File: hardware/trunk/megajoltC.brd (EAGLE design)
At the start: 79.9 x 63 mm, 116 parts, among them IC1 IC_FT230X-SSOP-16, IC2 MCP1826, IC3 MCP1826, J3 JUMPER_CLOSEDTHICK, U1 MCP1700, U11 TLV274, U12 PESDXS4UD, U18 MCP2551SO8, U4 ZXMS6004FF, U8 FAN8303, X1 MINI_USB_SHIELD, X3 MOLEX_MINIFIT-22

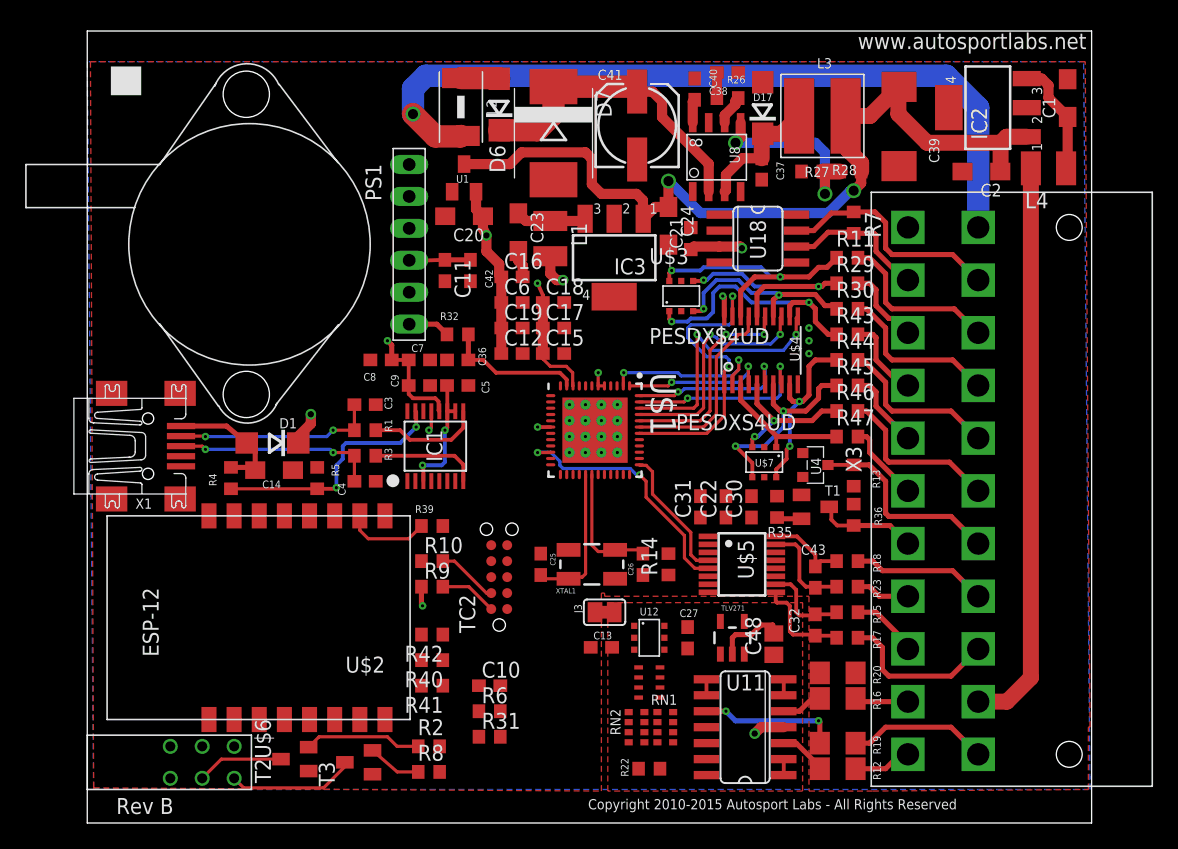
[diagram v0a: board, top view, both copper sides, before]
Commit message: Schematic, second draft complete
Also added gitignore
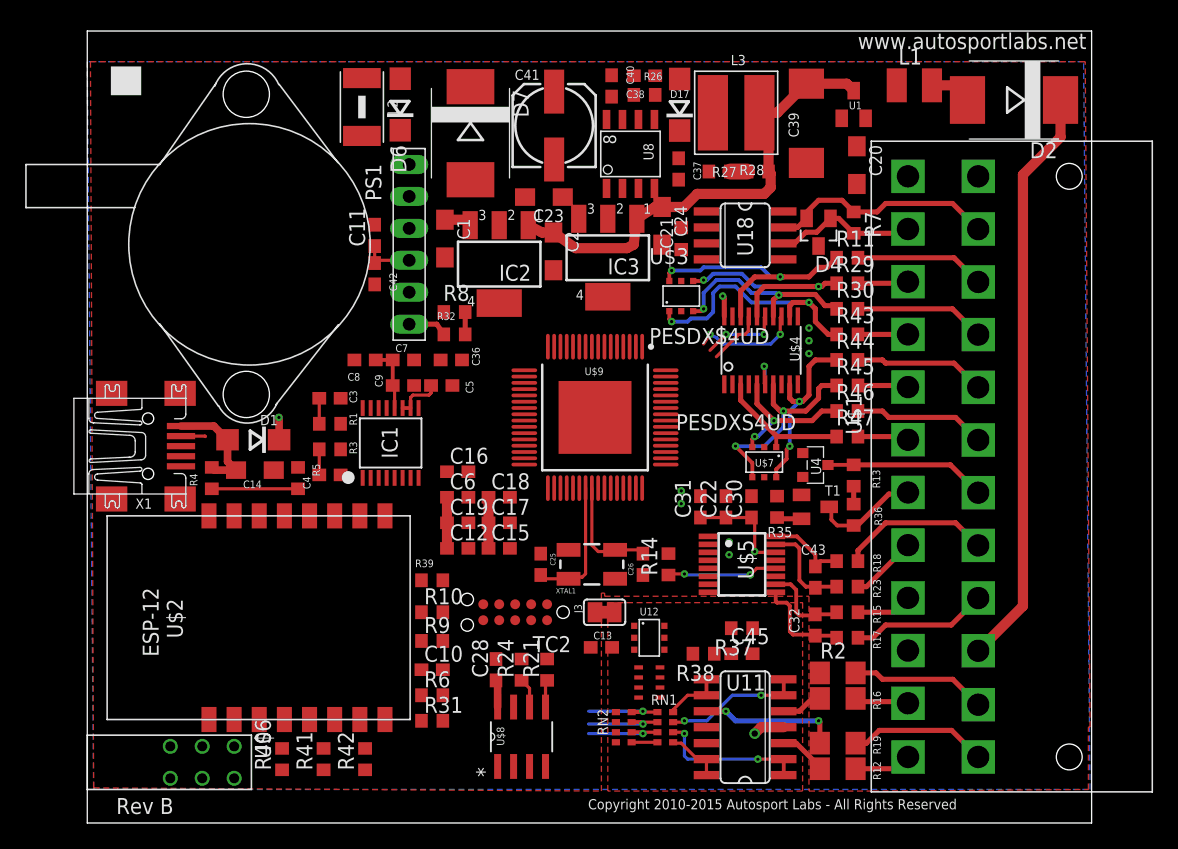
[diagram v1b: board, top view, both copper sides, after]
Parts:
- removed C27: .1uf, resistor:C0603
- removed C48: 0.1uF, rcl:C0805
- removed L4: 1uH, smt_inductors:1210
- removed R20: 10K, rcl:R1206
- removed R22: 2.1k, resistor:R0603
- removed T2, T3: (no value), transistor:SOT23-EBC
- removed TLV271: TLV271, texas_instruments:SOT23-5
- removed X3: MOLEX_MINIFIT-22, molex_mini-fit:MOLEX_MINIFIT-22
- added C28: .1uf, resistor:C0603
- added C45: .1uf, rcl:C0603
- added D2: (no value), diode:SMC
- added D4: PESD1CAN, diode:SOT23
- added R21, R24: 10k, resistor:R0603
- added R37: 43K 1%, rcl:R0603
- added R38: 10K 1%, rcl:R0603
- added U$8: 24LC64-I/SN, element14_microchip:SOIC127P600X175-8N
- added U$9: XMC4200F64K256QFP64, infineon_xmc:INF-PG-LQFP-64-5800X5800T28
- R2: device rcl:R0603 -> rcl:R1206
- R28: value 2.94K 1% -> 2.7K 1%
- R32: value 270 -> 5.6k
- R8: value 10K -> 10k
- U$1: value INF-PG-VQFN-48-53-5200X5200TE5 -> MOLEX_MINIFIT-JR-24; device infineon_xmc:INF-PG-VQFN-48-53-5200X5200TE5PRIMARY -> molex_mini-fit:MOLEX_MINIFIT-JR-24
- moved C1 50.8 mm to (28.4, 46.5), turned to 270 degrees
- moved IC2 40.8 mm to (32.8, 44.5), turned to 180 degrees
- moved R8 36.6 mm to (29.2, 40.6)
- moved C2 34.6 mm to (37.1, 45.5), turned to 270 degrees
- moved R2 33.0 mm to (59.7, 11.9)
- moved U$1 32.8 mm to (73.2, 30.5)
- moved U1 31.5 mm to (61.0, 57.1)
- moved C20 31.5 mm to (61.2, 52.3), turned to 270 degrees
- moved L1 31.4 mm to (65.8, 58.7), turned to 0 degrees
- moved C12 16.1 mm to (29.5, 21.8)
- moved C15 16.1 mm to (32.8, 21.8)
- moved C18 16.1 mm to (32.8, 25.9)
- moved C6 16.1 mm to (29.5, 25.9)
- moved C17 16.1 mm to (32.8, 23.9)
- moved C16 16.1 mm to (29.5, 27.9)
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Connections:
- removed net ANALOG-FREQ_1_OPAMP_OUT4: RN1.4, TLV271.1, TLV271.4
- removed net N$5: R8.1, T3.B
- removed net N$53: C1.+, IC2.3, L4.1
- removed net N$56: C23.+, IC3.3, L1.1
- removed net PROC_STATUS_LED_OUT1: T2.C, U$6.4
- removed net PROC_STATUS_LED_OUT2: T3.C, U$6.6
- new net AUX_ADC: RN1.4, RN2.5, U$9.19
- new net AUX_IN: R2.2, U$1.P14
- new net EEPROM_SCL: R24.1, U$8.6, U$9.59
- new net EEPROM_SDA: R21.1, U$8.5, U$9.62
- new net N$14: RN1.5, U11.13, U11.14
- new net UNUSED: U$1.P10
- new net VCC: C1.+, IC2.3, R31.2, R6.2, U$2.16
- net +3V3: now also C28.1, R21.2, R24.2, R40.1, R41.1, R42.1, U$8.8, U$9.13, U$9.22, U$9.38, U$9.42, U$9.56, U$9.8, U$9.9; no longer R31.2, R6.2, U$1.10, U$1.18, U$1.28, U$1.31, U$1.41, U$1.5, U$1.6, U$2.16
- net +5V: now also C23.+, IC3.3, L1.1; no longer L1.2, R40.1, R41.1, R42.1
- net AGND: now also C45.2, CN2.6, R38.2, RN2.4, U$9.21; no longer C27.2, C48.2, R22.1, TLV271.2, U$1.17
- net CAM_TIM_IN: now also U$9.30; no longer U$1.22
- net CAM_VRS+: now also U$1.P16; no longer X3.P14
- net CAM_VRS-: now also U$1.P9; no longer X3.P9
- net CANH: now also D4.2, U$1.P23; no longer X3.P21
- net CANL: now also D4.1, U$1.P2; no longer X3.P2
- net CAN_RX: now also U$9.36; no longer U$1.15
- net CAN_TX: now also U$9.34, U$9.35; no longer U$1.26
- net CLT_ADC: now also U$9.20; no longer U$1.16
- net CLT_IN: now also U$1.P12; no longer X3.P11
- net COIL1: now also U$1.P22; no longer X3.P20
- net COIL2: now also U$1.P3; no longer X3.P3
- net COIL3: now also U$1.P21; no longer X3.P19
- net COIL4: now also U$1.P4; no longer X3.P4
- net COIL5: now also U$1.P20; no longer X3.P18
- net COIL6: now also U$1.P5; no longer X3.P5
- net COIL7: now also U$1.P19; no longer X3.P17
- net COIL8: now also U$1.P6; no longer X3.P6
- net CRANK_TIM_IN: now also U$9.28; no longer U$1.37
- net CRANK_VRS+: now also U$1.P17; no longer X3.P15
- net CRANK_VRS-: now also U$1.P8; no longer X3.P8
- net ESP_GPIO0: now also U$9.49
- net ESP_RXD: now also U$9.29; no longer U$1.21
- net ESP_TXD: now also U$9.32; no longer U$1.24
- net FTDI_RXD: now also U$9.47; no longer U$1.35
- net FTDI_TXD: now also U$9.48; no longer U$1.36
- net GND: now also C28.2, D4.3, R8.1, U$1.P1, U$8.1, U$8.2, U$8.3, U$8.4, U$9.37, U$9.41, U$9.65; no longer T2.E, T3.E, U$1.27, U$1.49, X3.P1
- net GPO_COIL1: now also U$9.2; no longer U$1.2
- net GPO_COIL2: now also U$9.1; no longer U$1.1
- net GPO_COIL3: now also U$9.64; no longer U$1.48
- net GPO_COIL4: now also U$9.63; no longer U$1.47
- net GPO_COIL5: now also U$9.61; no longer U$1.46
- net GPO_COIL6: now also U$9.60; no longer U$1.45
- net GPO_COIL7: now also U$9.58; no longer U$1.44
- net GPO_COIL8: now also U$9.57; no longer U$1.43
- net GPO_COIL_EN: now also U$9.4; no longer U$1.42
- net IAT_ADC: now also U$9.18; no longer U$1.14
- net IAT_IN: now also U$1.P13; no longer X3.P12
- net MAP_ADC: now also R8.2, U$9.15; no longer U$1.11
- net N$2: now also D2.A, L1.2; no longer R2.1, T2.B
- net N$21: now also U$9.40; no longer U$1.30
- net N$25: now also U$9.39; no longer U$1.29
- net N$31: now also CN2.3, R2.1, U11.12; no longer C48.1, R20.1, TLV271.3
- net PGM_GPO: now also U$9.31; no longer U$1.23
- net PGM_OUT: now also U$1.P18; no longer X3.P16
- net RAW_+12V: now also U$1.P24; no longer X3.P22
- net SAFE_+12V: now also R37.1; no longer C27.1, R20.2, TLV271.5
- net STATUS_LED_1: now also U$6.4, U$9.27; no longer R2.2, U$1.20
- net STATUS_LED_2: now also U$6.6, U$9.26; no longer R8.2, U$1.19
- net SWCLK: now also U$9.45; no longer U$1.34
- net SWDIO: now also U$9.44; no longer U$1.33
- net TACH_GPO: now also U$9.33; no longer U$1.25
- net TACH_OUT: now also U$1.P7; no longer X3.P7
- net TPS_ADC: now also U$9.17; no longer U$1.13
- net TPS_IN: now also U$1.P11; no longer X3.P10
- net VBATT_ADC: now also C45.1, R37.2, R38.1, U$9.16; no longer R22.2, RN1.5, U$1.12
- net VREF: now also D2.C, U$1.P15; no longer L4.2, X3.P13
- net XMC_RESET: now also U$9.43; no longer U$1.32
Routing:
- net RAW_+12V: track 62.5 -> 0.00 mm, vias 1 -> 0
- net VDD: track 67.6 -> 37.6 mm, vias 2 -> 0
- net GPO_COIL_EN: track 24.2 -> 0.00 mm, vias 2 -> 0
- net SAFE_+12V: track 24.9 -> 1.42 mm
- net +3V3: track 36.9 -> 15.5 mm, vias 6 -> 0
- net GPO_COIL5: track 20.9 -> 0.00 mm, vias 2 -> 0
- net CAM_TIM_IN: track 20.4 -> 0.00 mm, vias 2 -> 0
- net GPO_COIL4: track 15.2 -> 0.00 mm, vias 2 -> 0
- net N$8: track 15.7 -> 1.35 mm, vias 2 -> 0
- net FTDI_DP: track 16.1 -> 2.03 mm, vias 2 -> 0
- net GPO_COIL1: track 13.4 -> 0.00 mm, vias 2 -> 0
- net FTDI_VBUS_SENSE: track 19.7 -> 6.86 mm, vias 2 -> 0
- net FTDI_DM: track 16.0 -> 3.99 mm, vias 2 -> 0
- net GPO_COIL2: track 11.8 -> 0.00 mm, vias 2 -> 0
- net GPO_COIL8: track 15.7 -> 4.57 mm
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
